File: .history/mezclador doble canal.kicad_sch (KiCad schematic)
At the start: 31 parts, among them J1 Conn_Coaxial, J2 Conn_Coaxial, J3 Conn_Coaxial, J4 Conn_Coaxial, J5 Conn_Coaxial, J6 Conn_Coaxial, U1 NE5532

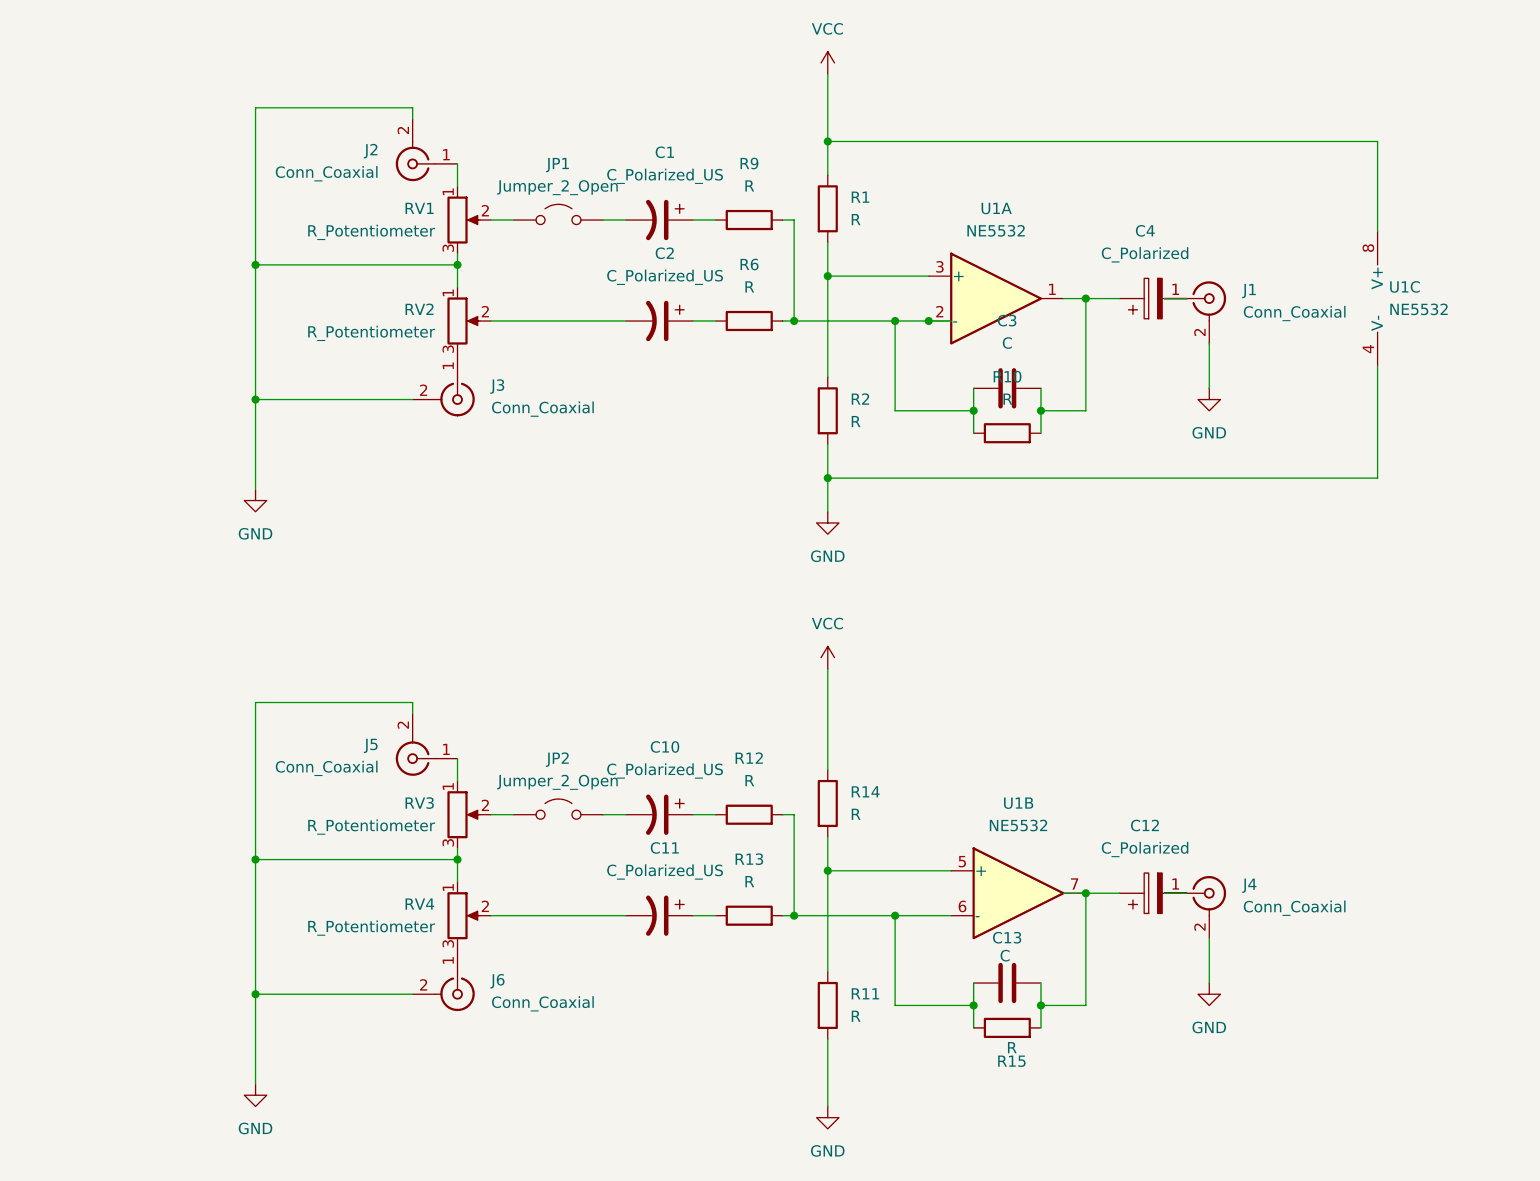
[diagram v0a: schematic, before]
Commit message: trabajando canal R
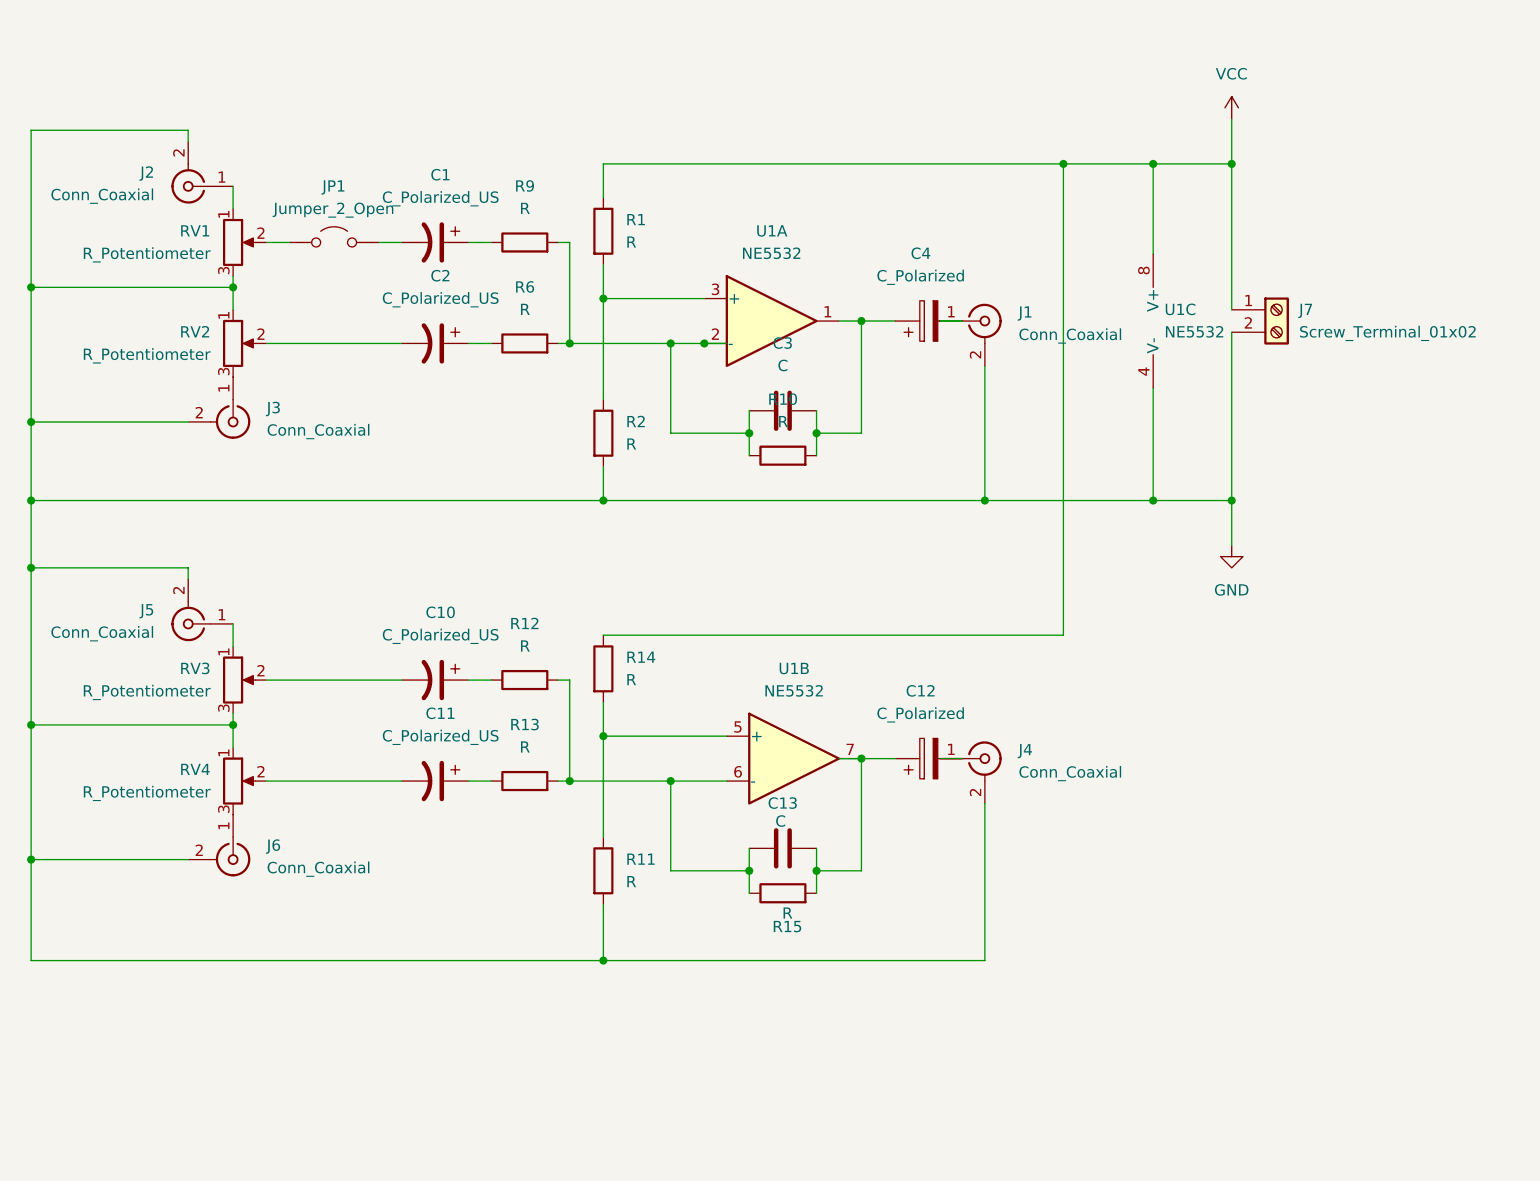
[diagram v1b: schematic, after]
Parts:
- removed JP2: Jumper_2_Open, personal:Jumper_Wire_10mm, symbol Jumper:Jumper_2_Open
- added J7: Screw_Terminal_01x02, Connector:JWT_A3963_1x02_P3.96mm_Vertical, symbol Connector:Screw_Terminal_01x02
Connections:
- net GND: now also J7.2 (Pin_2)
- net VCC: now also J7.1 (Pin_1)
- net at RV3.2: now also C10.2
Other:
- moved on the sheet: C1, C10, C11, C12, C13, C2, C3, C4, J1, J2, J3, J4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
